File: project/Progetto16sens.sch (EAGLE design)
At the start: 128 parts, among them IC1 LMZ14202TZE-ADJ_NOPB, J2 455-1750-1-ND, M1 43650-0201, M2 43650-0201, M3 43650-0201, M4 43650-0201, M5 ARDUINO-PRO-MINI

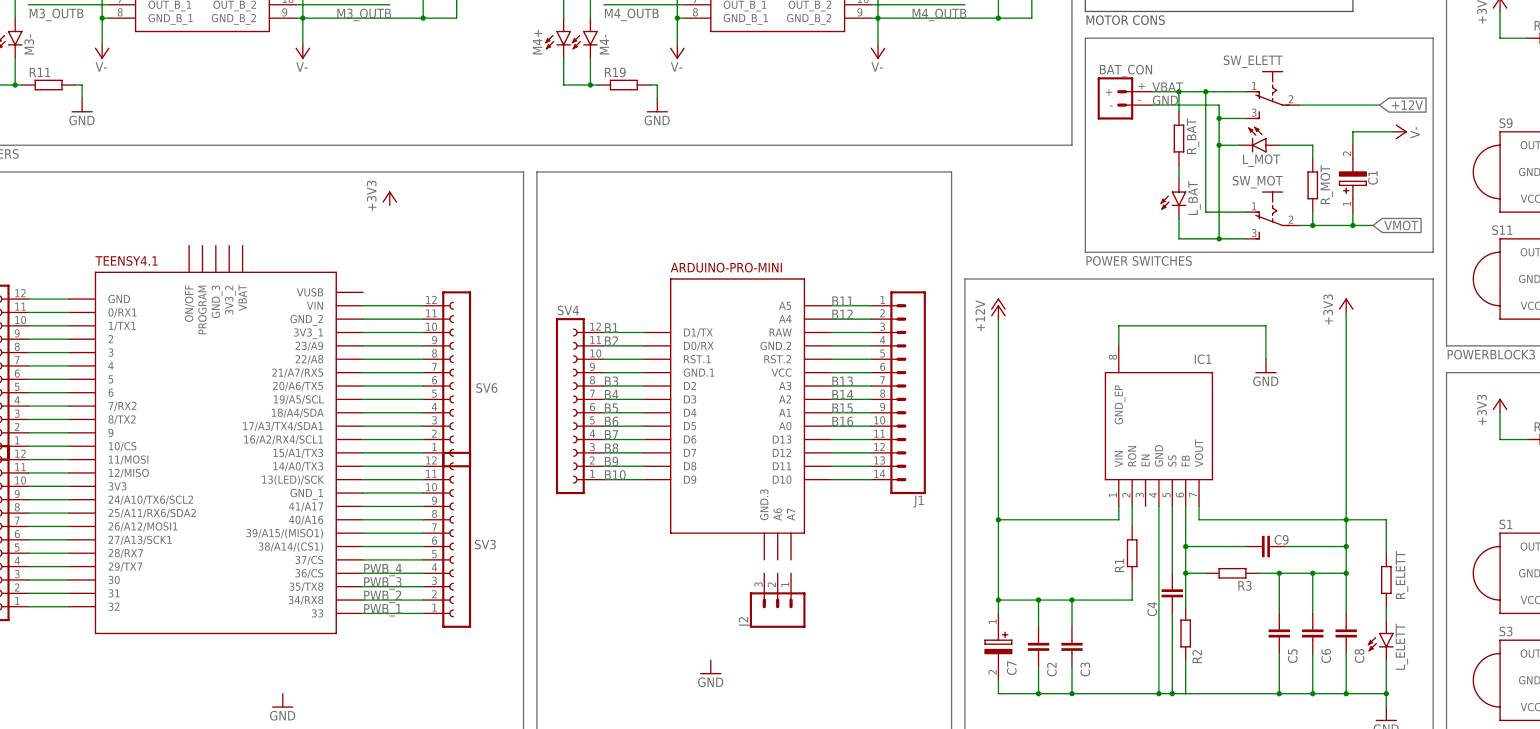
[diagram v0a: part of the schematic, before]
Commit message: greve
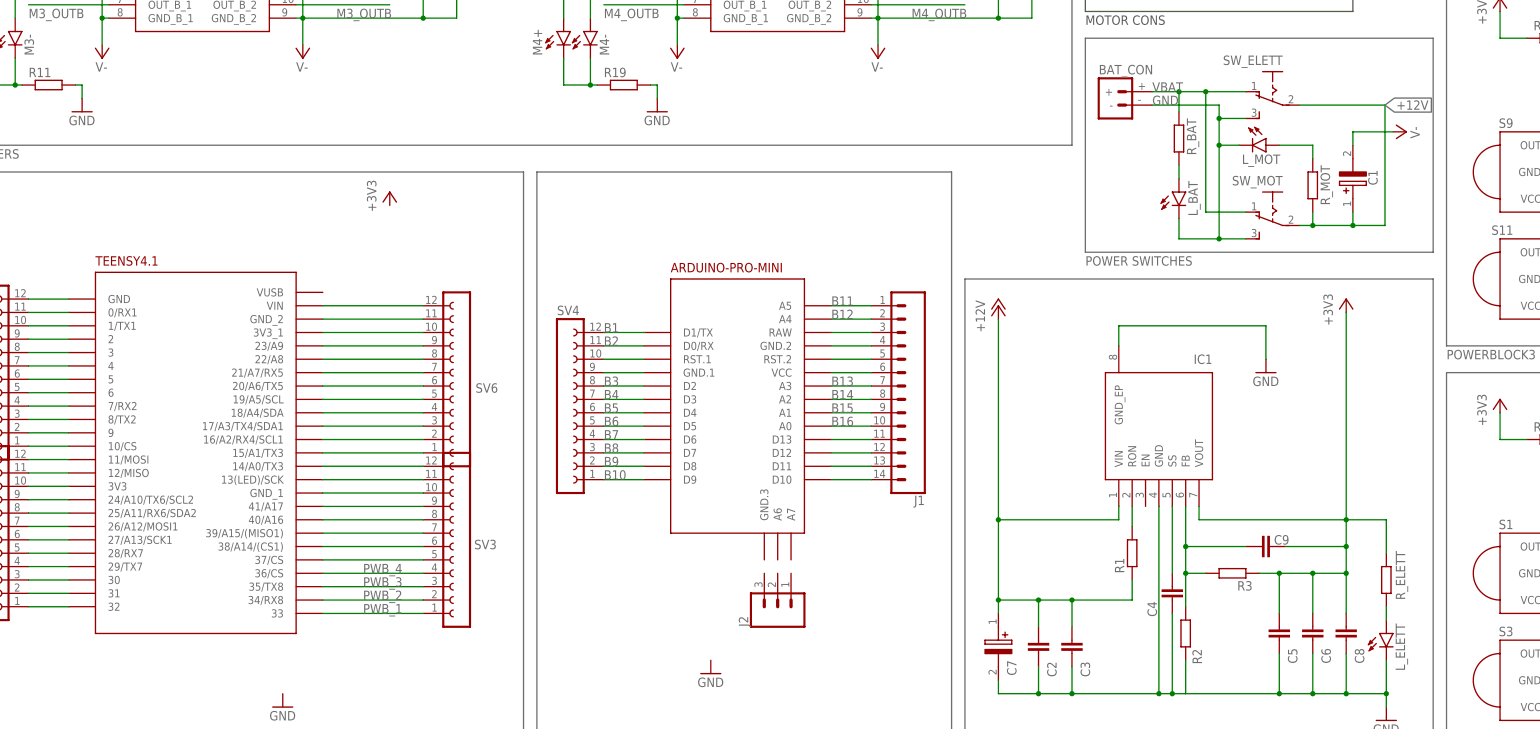
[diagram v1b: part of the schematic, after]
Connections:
- removed net VMOT: C1.+, R_MOT.2, SW_MOT.P
- net +12V: now also C1.+, R_MOT.2, SW_MOT.P
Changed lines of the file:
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@@
-</segment>
-</net>
-<net name="VMOT" class="0">
-<segment>
-<pinref part="SW_MOT" gate="1" pin="P"/>
-<wire x1="261.62" y1="101.6" x2="264.16" y2="101.6" width="0.1524" layer="91"/>
-<pinref part="R_MOT" gate="G$1" pin="2"/>
-<wire x1="264.16" y1="101.6" x2="271.78" y2="101.6" width="0.1524" layer="91"/>
-<wire x1="271.78" y1="101.6" x2="275.59" y2="101.6" width="0.1524" layer="91"/>
-<wire x1="264.16" y1="104.14" x2="264.16" y2="101.6" width="0.1524" layer="91"/>
-<junction x="264.16" y="101.6"/>
-<pinref part="C1" gate="G$1" pin="+"/>
-<wire x1="271.78" y1="104.14" x2="271.78" y2="101.6" width="0.1524" layer="91"/>
-<junction x="271.78" y="101.6"/>
-<label x="275.59" y="101.6" size="1.778" layer="95" xref="yes"/>
 </segment>
 </net>
@@
 </net>
 <net name="+12V" class="0">
-<segment>
-<pinref part="SW_ELETT" gate="1" pin="P"/>
-<wire x1="261.62" y1="124.46" x2="276.86" y2="124.46" width="0.1524" layer="91"/>
-<label x="276.86" y="124.46" size="1.778" layer="95" xref="yes"/>
-</segment>
 <segment>
 <pinref part="IC1" gate="G$1" pin="VIN"/>
@@
 <junction x="204.47" y="161.29"/>
 </segment>
+<segment>
+<pinref part="SW_MOT" gate="1" pin="P"/>
+<wire x1="261.62" y1="101.6" x2="264.16" y2="101.6" width="0.1524" layer="91"/>
+<pinref part="R_MOT" gate="G$1" pin="2"/>
+<wire x1="264.16" y1="101.6" x2="271.78" y2="101.6" width="0.1524" layer="91"/>
+<wire x1="264.16" y1="104.14" x2="264.16" y2="101.6" width="0.1524" layer="91"/>
+<junction x="264.16" y="101.6"/>
+<pinref part="C1" gate="G$1" pin="+"/>
+<wire x1="271.78" y1="104.14" x2="271.78" y2="101.6" width="0.1524" layer="91"/>
+<junction x="271.78" y="101.6"/>
+<pinref part="SW_ELETT" gate="1" pin="P"/>
+<wire x1="261.62" y1="124.46" x2="277.876" y2="124.46" width="0.1524" layer="91"/>
+<label x="277.876" y="124.46" size="1.778" layer="95" xref="yes"/>
+<wire x1="271.78" y1="101.6" x2="277.876" y2="101.6" width="0.1524" layer="91"/>
+<wire x1="277.876" y1="101.6" x2="277.876" y2="124.46" width="0.1524" layer="91"/>
+</segment>
 </net>
 <net name="N$6" class="0">
@@
 <pinref part="U$1" gate="G$1" pin="34/RX8"/>
 <pinref part="SV3" gate="G$1" pin="2"/>
-<wire x1="83.82" y1="30.48" x2="95.25" y2="30.48" width="0.1524" layer="91"/>
+<wire x1="76.2" y1="30.48" x2="95.25" y2="30.48" width="0.1524" layer="91"/>
 <label x="83.82" y="30.48" size="1.778" layer="95"/>
 </segment>
@@
 <pinref part="U$1" gate="G$1" pin="33"/>
 <pinref part="SV3" gate="G$1" pin="1"/>
-<wire x1="83.82" y1="27.94" x2="95.25" y2="27.94" width="0.1524" layer="91"/>
+<wire x1="76.2" y1="27.94" x2="95.25" y2="27.94" width="0.1524" layer="91"/>
 <label x="83.82" y="27.94" size="1.778" layer="95"/>
 </segment>
@@
 <pinref part="U$1" gate="G$1" pin="35/TX8"/>
 <pinref part="SV3" gate="G$1" pin="3"/>
-<wire x1="83.82" y1="33.02" x2="95.25" y2="33.02" width="0.1524" layer="91"/>
+<wire x1="76.2" y1="33.02" x2="95.25" y2="33.02" width="0.1524" layer="91"/>
 <label x="83.82" y="33.02" size="1.778" layer="95"/>
 </segment>
@@
 <pinref part="U$1" gate="G$1" pin="36/CS"/>
 <pinref part="SV3" gate="G$1" pin="4"/>
-<wire x1="83.82" y1="35.56" x2="95.25" y2="35.56" width="0.1524" layer="91"/>
+<wire x1="76.2" y1="35.56" x2="95.25" y2="35.56" width="0.1524" layer="91"/>
 <label x="83.82" y="35.56" size="1.778" layer="95"/>
 </segment>
@@
 <pinref part="U$1" gate="G$1" pin="VIN"/>
 <pinref part="SV6" gate="G$1" pin="12"/>
-<wire x1="83.82" y1="86.36" x2="95.25" y2="86.36" width="0.1524" layer="91"/>
+<wire x1="76.2" y1="86.36" x2="95.25" y2="86.36" width="0.1524" layer="91"/>
 </segment>
 </net>
@@
 <pinref part="U$1" gate="G$1" pin="23/A9"/>
 <pinref part="SV6" gate="G$1" pin="9"/>
-<wire x1="83.82" y1="78.74" x2="95.25" y2="78.74" width="0.1524" layer="91"/>
+<wire x1="76.2" y1="78.74" x2="95.25" y2="78.74" width="0.1524" layer="91"/>
 </segment>
 </net>
@@
 <pinref part="U$1" gate="G$1" pin="22/A8"/>
 <pinref part="SV6" gate="G$1" pin="8"/>
-<wire x1="83.82" y1="76.2" x2="95.25" y2="76.2" width="0.1524" layer="91"/>
+<wire x1="76.2" y1="76.2" x2="95.25" y2="76.2" width="0.1524" layer="91"/>
 </segment>
 </net>
@@
 <pinref part="U$1" gate="G$1" pin="21/A7/RX5"/>
 <pinref part="SV6" gate="G$1" pin="7"/>
-<wire x1="83.82" y1="73.66" x2="95.25" y2="73.66" width="0.1524" layer="91"/>
+<wire x1="76.2" y1="73.66" x2="95.25" y2="73.66" width="0.1524" layer="91"/>
 </segment>
 </net>
@@
 <segment>
 <pinref part="U$1" gate="G$1" pin="20/A6/TX5"/>
-<wire x1="83.82" y1="71.12" x2="95.25" y2="71.12" width="0.1524" layer="91"/>
+<wire x1="76.2" y1="71.12" x2="95.25" y2="71.12" width="0.1524" layer="91"/>
 <pinref part="SV6" gate="G$1" pin="6"/>
 </segment>
@@
 <pinref part="U$1" gate="G$1" pin="19/A5/SCL"/>
 <pinref part="SV6" gate="G$1" pin="5"/>
-<wire x1="83.82" y1="68.58" x2="95.25" y2="68.58" width="0.1524" layer="91"/>
+<wire x1="76.2" y1="68.58" x2="95.25" y2="68.58" width="0.1524" layer="91"/>
 </segment>
 </net>
@@
 <pinref part="U$1" gate="G$1" pin="18/A4/SDA"/>
 <pinref part="SV6" gate="G$1" pin="4"/>
-<wire x1="83.82" y1="66.04" x2="95.25" y2="66.04" width="0.1524" layer="91"/>
+<wire x1="76.2" y1="66.04" x2="95.25" y2="66.04" width="0.1524" layer="91"/>
 </segment>
 </net>
@@
 <pinref part="U$1" gate="G$1" pin="17/A3/TX4/SDA1"/>
 <pinref part="SV6" gate="G$1" pin="3"/>
-<wire x1="83.82" y1="63.5" x2="95.25" y2="63.5" width="0.1524" layer="91"/>
+<wire x1="76.2" y1="63.5" x2="95.25" y2="63.5" width="0.1524" layer="91"/>
 </segment>
 </net>
@@
 <pinref part="U$1" gate="G$1" pin="16/A2/RX4/SCL1"/>
 <pinref part="SV6" gate="G$1" pin="2"/>
-<wire x1="83.82" y1="60.96" x2="95.25" y2="60.96" width="0.1524" layer="91"/>
+<wire x1="76.2" y1="60.96" x2="95.25" y2="60.96" width="0.1524" layer="91"/>
 </segment>
 </net>
@@
 <pinref part="U$1" gate="G$1" pin="15/A1/TX3"/>
 <pinref part="SV6" gate="G$1" pin="1"/>
-<wire x1="83.82" y1="58.42" x2="95.25" y2="58.42" width="0.1524" layer="91"/>
+<wire x1="76.2" y1="58.42" x2="95.25" y2="58.42" width="0.1524" layer="91"/>
 </segment>
 </net>
@@
 <pinref part="U$1" gate="G$1" pin="14/A0/TX3"/>
 <pinref part="SV3" gate="G$1" pin="12"/>
-<wire x1="83.82" y1="55.88" x2="95.25" y2="55.88" width="0.1524" layer="91"/>
+<wire x1="76.2" y1="55.88" x2="95.25" y2="55.88" width="0.1524" layer="91"/>
 </segment>
 </net>
@@
 <pinref part="U$1" gate="G$1" pin="13(LED)/SCK"/>
 <pinref part="SV3" gate="G$1" pin="11"/>
-<wire x1="83.82" y1="53.34" x2="95.25" y2="53.34" width="0.1524" layer="91"/>
+<wire x1="76.2" y1="53.34" x2="95.25" y2="53.34" width="0.1524" layer="91"/>
 </segment>
 </net>
@@
 <pinref part="U$1" gate="G$1" pin="41/A17"/>
 <pinref part="SV3" gate="G$1" pin="9"/>
-<wire x1="83.82" y1="48.26" x2="95.25" y2="48.26" width="0.1524" layer="91"/>
+<wire x1="76.2" y1="48.26" x2="95.25" y2="48.26" width="0.1524" layer="91"/>
 </segment>
 </net>
@@
 <pinref part="U$1" gate="G$1" pin="40/A16"/>
 <pinref part="SV3" gate="G$1" pin="8"/>
-<wire x1="83.82" y1="45.72" x2="95.25" y2="45.72" width="0.1524" layer="91"/>
+<wire x1="76.2" y1="45.72" x2="95.25" y2="45.72" width="0.1524" layer="91"/>
 </segment>
 </net>
@@
 <pinref part="U$1" gate="G$1" pin="38/A14/(CS1)"/>
 <pinref part="SV3" gate="G$1" pin="6"/>
-<wire x1="83.82" y1="40.64" x2="95.25" y2="40.64" width="0.1524" layer="91"/>
+<wire x1="76.2" y1="40.64" x2="95.25" y2="40.64" width="0.1524" layer="91"/>
 </segment>
 </net>
@@
 <segment>
 <pinref part="U$1" gate="G$1" pin="39/A15/(MISO1)"/>
-<wire x1="83.82" y1="43.18" x2="95.25" y2="43.18" width="0.1524" layer="91"/>
+<wire x1="76.2" y1="43.18" x2="95.25" y2="43.18" width="0.1524" layer="91"/>
 <pinref part="SV3" gate="G$1" pin="7"/>
 </segment>
@@
 <segment>
 <pinref part="U$1" gate="G$1" pin="37/CS"/>
-<wire x1="83.82" y1="38.1" x2="95.25" y2="38.1" width="0.1524" layer="91"/>
+<wire x1="76.2" y1="38.1" x2="95.25" y2="38.1" width="0.1524" layer="91"/>
 <pinref part="SV3" gate="G$1" pin="5"/>
 </segment>
@@
 <pinref part="U$1" gate="G$1" pin="3V3_1"/>
 <pinref part="SV6" gate="G$1" pin="10"/>
-<wire x1="83.82" y1="81.28" x2="95.25" y2="81.28" width="0.1524" layer="91"/>
+<wire x1="76.2" y1="81.28" x2="95.25" y2="81.28" width="0.1524" layer="91"/>
 </segment>
 </net>
@@
 <pinref part="SV6" gate="G$1" pin="11"/>
 <pinref part="U$1" gate="G$1" pin="GND_2"/>
-<wire x1="83.82" y1="83.82" x2="95.25" y2="83.82" width="0.1524" layer="91"/>
+<wire x1="76.2" y1="83.82" x2="95.25" y2="83.82" width="0.1524" layer="91"/>
 </segment>
 </net>
@@
 <pinref part="SV3" gate="G$1" pin="10"/>
 <pinref part="U$1" gate="G$1" pin="GND_1"/>
-<wire x1="83.82" y1="50.8" x2="95.25" y2="50.8" width="0.1524" layer="91"/>
-</segment>
-</net>
+<wire x1="76.2" y1="50.8" x2="95.25" y2="50.8" width="0.1524" layer="91"/>
+</segment>
+</net>
